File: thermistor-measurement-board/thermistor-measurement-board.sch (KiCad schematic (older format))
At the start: 0 parts

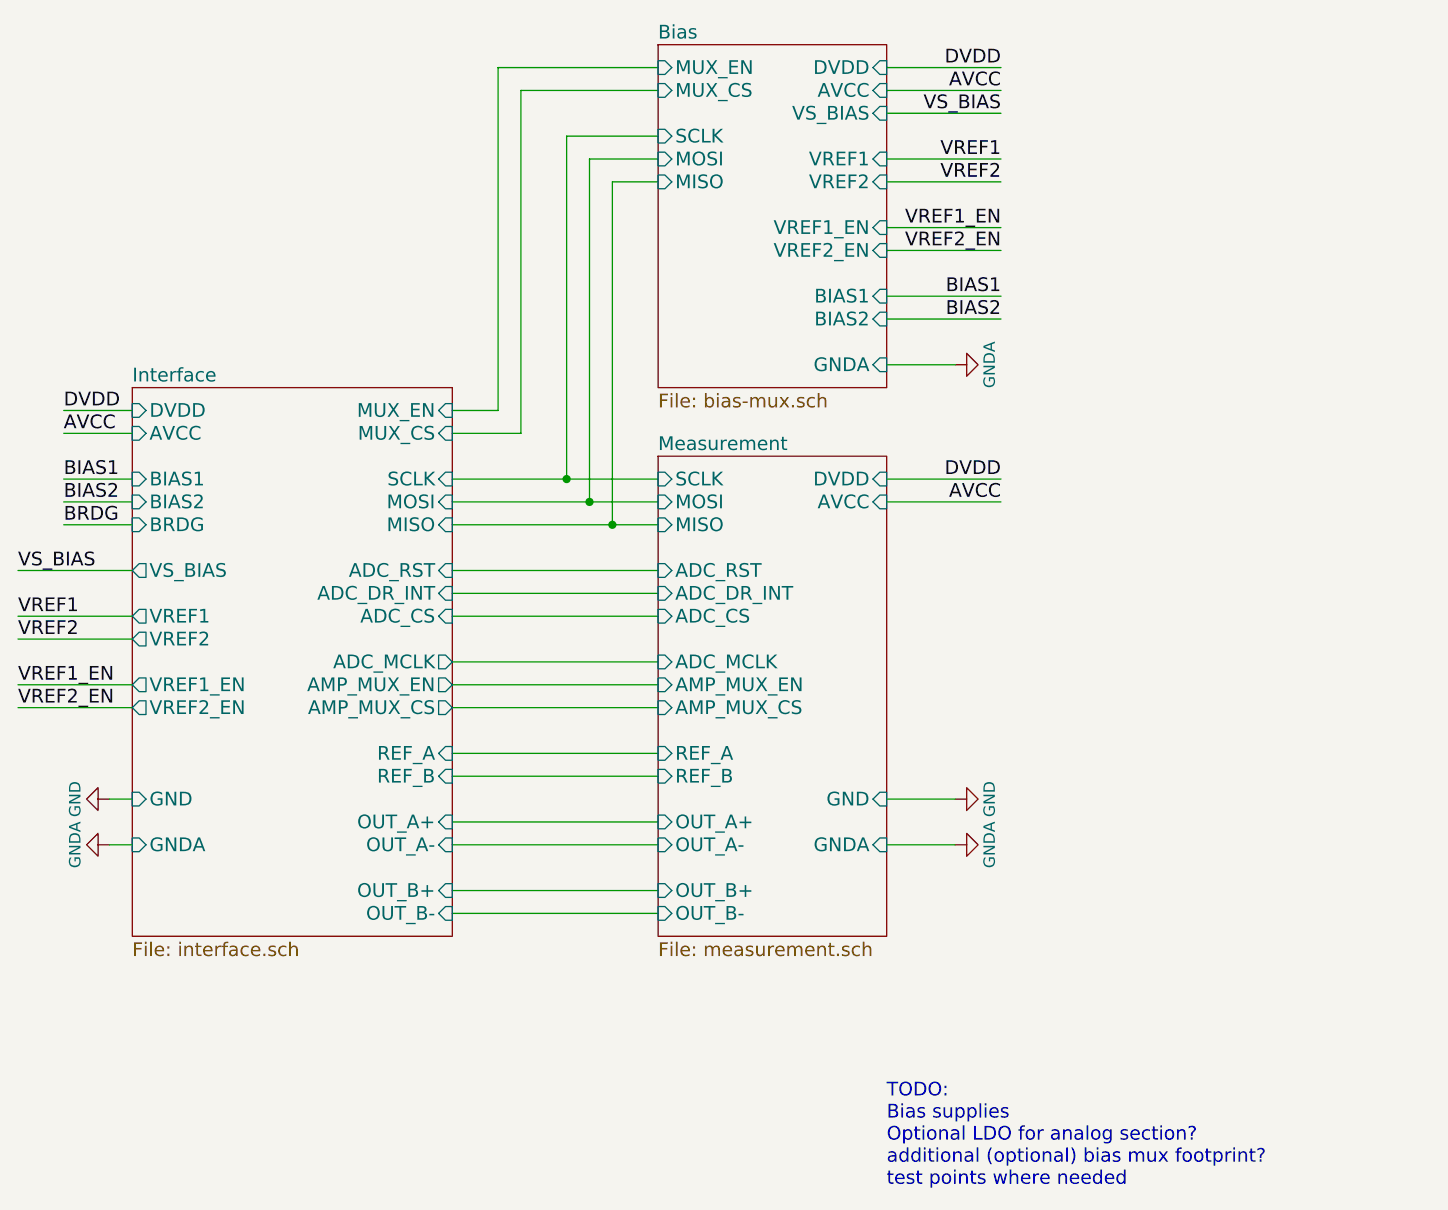
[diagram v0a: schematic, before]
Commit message: took care of a few board review tasks
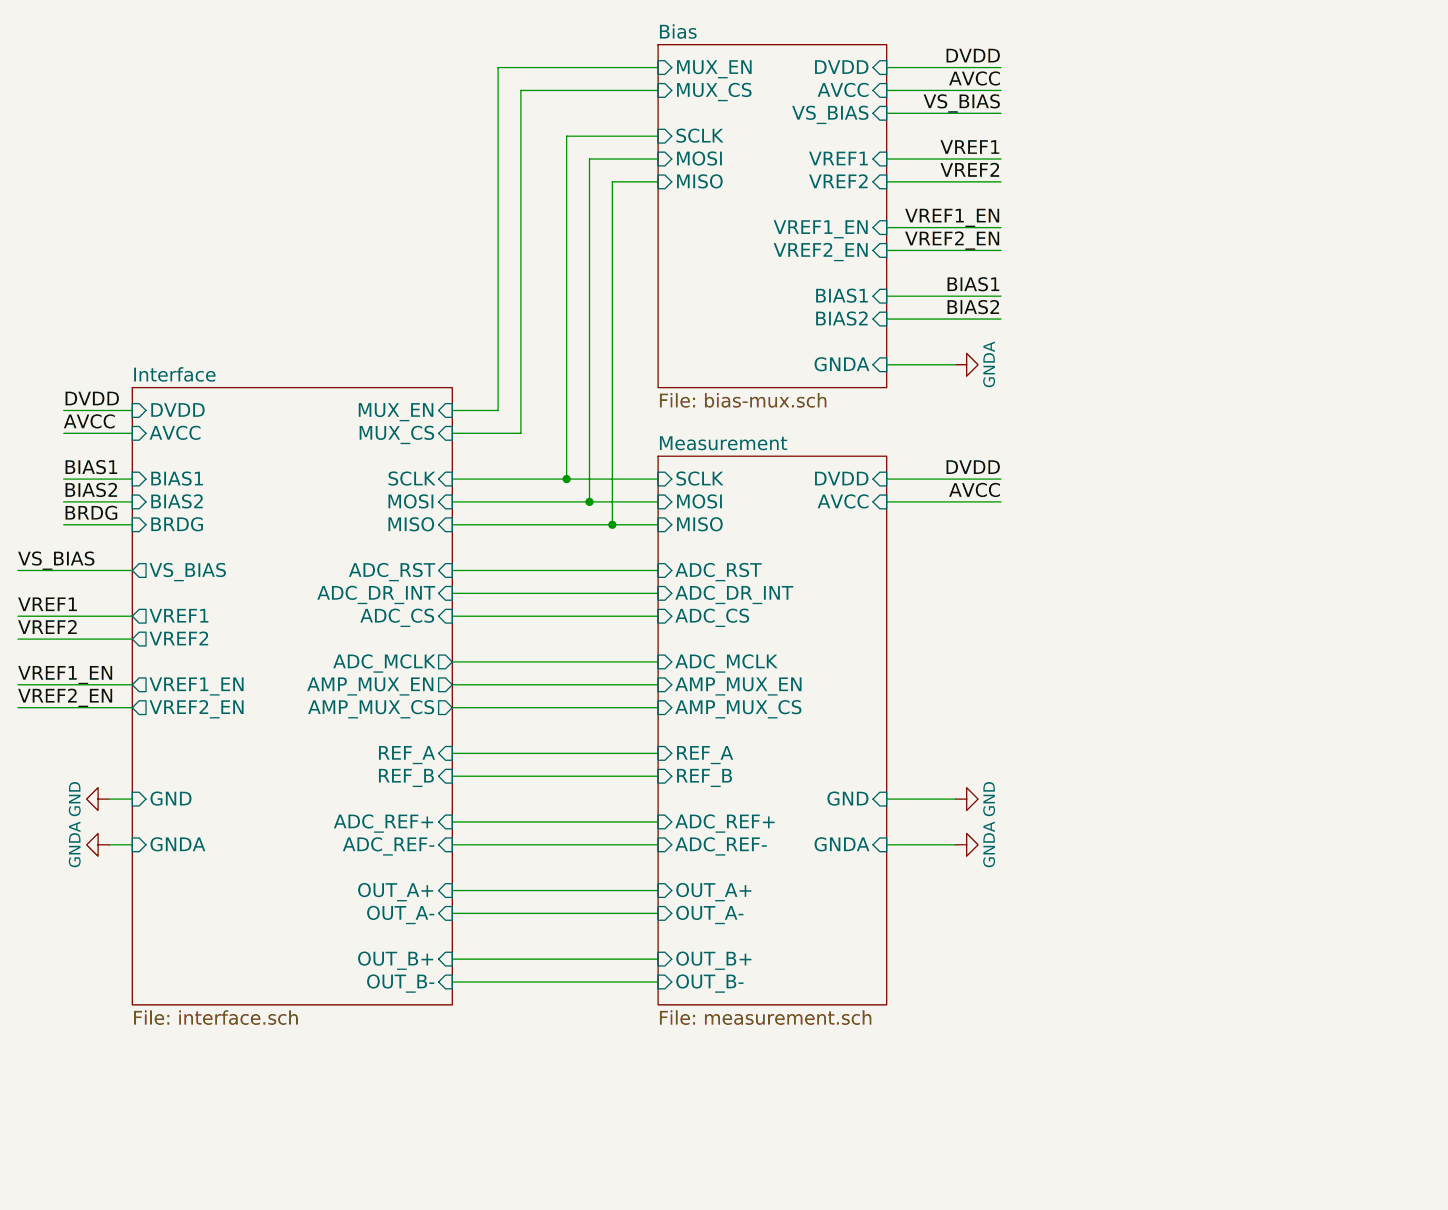
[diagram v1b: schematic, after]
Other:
- note removed: "TODO:\nBias supplies\nOptional LDO for analog section?\nadditional (optional) bias mux footprint?\ntest points where needed"
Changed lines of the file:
@@
 Comment4 ""
 $EndDescr
-Text Notes 7000 7100 0    60   ~ 0
-TODO:\nBias supplies\nOptional LDO for analog section?\nadditional (optional) bias mux footprint?\ntest points where needed
 $Sheet
 S 6000 2100 1000 1500
@@
 $EndSheet
 $Sheet
-S 6000 3900 1000 2100
+S 6000 3900 1000 2400
 U 56B5D807
 F0 "Measurement" 60
@@
 F10 "ADC_DR_INT" I L 6000 4500 60
 F11 "ADC_RST" I L 6000 4400 60
-F12 "OUT_B+" I L 6000 5800 60
-F13 "OUT_B-" I L 6000 5900 60
+F12 "OUT_B+" I L 6000 6100 60
+F13 "OUT_B-" I L 6000 6200 60
 F14 "AMP_MUX_CS" I L 6000 5000 60
 F15 "AMP_MUX_EN" I L 6000 4900 60
-F16 "OUT_A+" I L 6000 5500 60
-F17 "OUT_A-" I L 6000 5600 60
+F16 "OUT_A+" I L 6000 5800 60
+F17 "OUT_A-" I L 6000 5900 60
 F18 "ADC_MCLK" I L 6000 4800 60
 F19 "REF_A" I L 6000 5200 60
 F20 "REF_B" I L 6000 5300 60
+F21 "ADC_REF+" I L 6000 5500 60
+F22 "ADC_REF-" I L 6000 5600 60
 $EndSheet
 $Comp
@@
 $EndComp
 $Sheet
-S 3700 3600 1400 2400
+S 3700 3600 1400 2700
 U 56B64232
 F0 "Interface" 60
@@
 F15 "ADC_DR_INT" I R 5100 4500 60
 F16 "ADC_RST" I R 5100 4400 60
-F17 "OUT_A+" I R 5100 5500 60
-F18 "OUT_A-" I R 5100 5600 60
-F19 "OUT_B+" I R 5100 5800 60
-F20 "OUT_B-" I R 5100 5900 60
+F17 "OUT_A+" I R 5100 5800 60
+F18 "OUT_A-" I R 5100 5900 60
+F19 "OUT_B+" I R 5100 6100 60
+F20 "OUT_B-" I R 5100 6200 60
 F21 "AMP_MUX_CS" O R 5100 5000 60
 F22 "AMP_MUX_EN" O R 5100 4900 60
@@
 F29 "VREF2_EN" O L 3700 5000 60
 F30 "VREF1_EN" O L 3700 4900 60
+F31 "ADC_REF+" I R 5100 5500 60
+F32 "ADC_REF-" I R 5100 5600 60
 $EndSheet
 Text Label 7500 3200 2    60   ~ 0
@@
 	5100 5300 6000 5300
 Wire Wire Line
-	6000 5500 5100 5500
-Wire Wire Line
-	5100 5600 6000 5600
+	6000 5800 5100 5800
+Wire Wire Line
+	5100 5900 6000 5900
 Wire Wire Line
 	6000 5000 5100 5000
 Wire Wire Line
-	6000 5800 5100 5800
-Wire Wire Line
-	5100 5900 6000 5900
+	6000 6100 5100 6100
+Wire Wire Line
+	5100 6200 6000 6200
 Text Label 7500 2400 2    60   ~ 0
 VS_BIAS
@@
 Wire Wire Line
 	3700 4900 3200 4900
+Wire Wire Line
+	6000 5500 5100 5500
+Wire Wire Line
+	5100 5600 6000 5600
 $EndSCHEMATC
